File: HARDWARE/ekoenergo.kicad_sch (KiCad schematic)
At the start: 36 parts, among them J1 WSH500, J2 DC+, J3 EARTH, J4 DC-, J5 A, J6 B, Q1 47n60, Q2 47n60, Q3 47n60, Q4 47n60, U5 ACS712ELCTR-20A-T

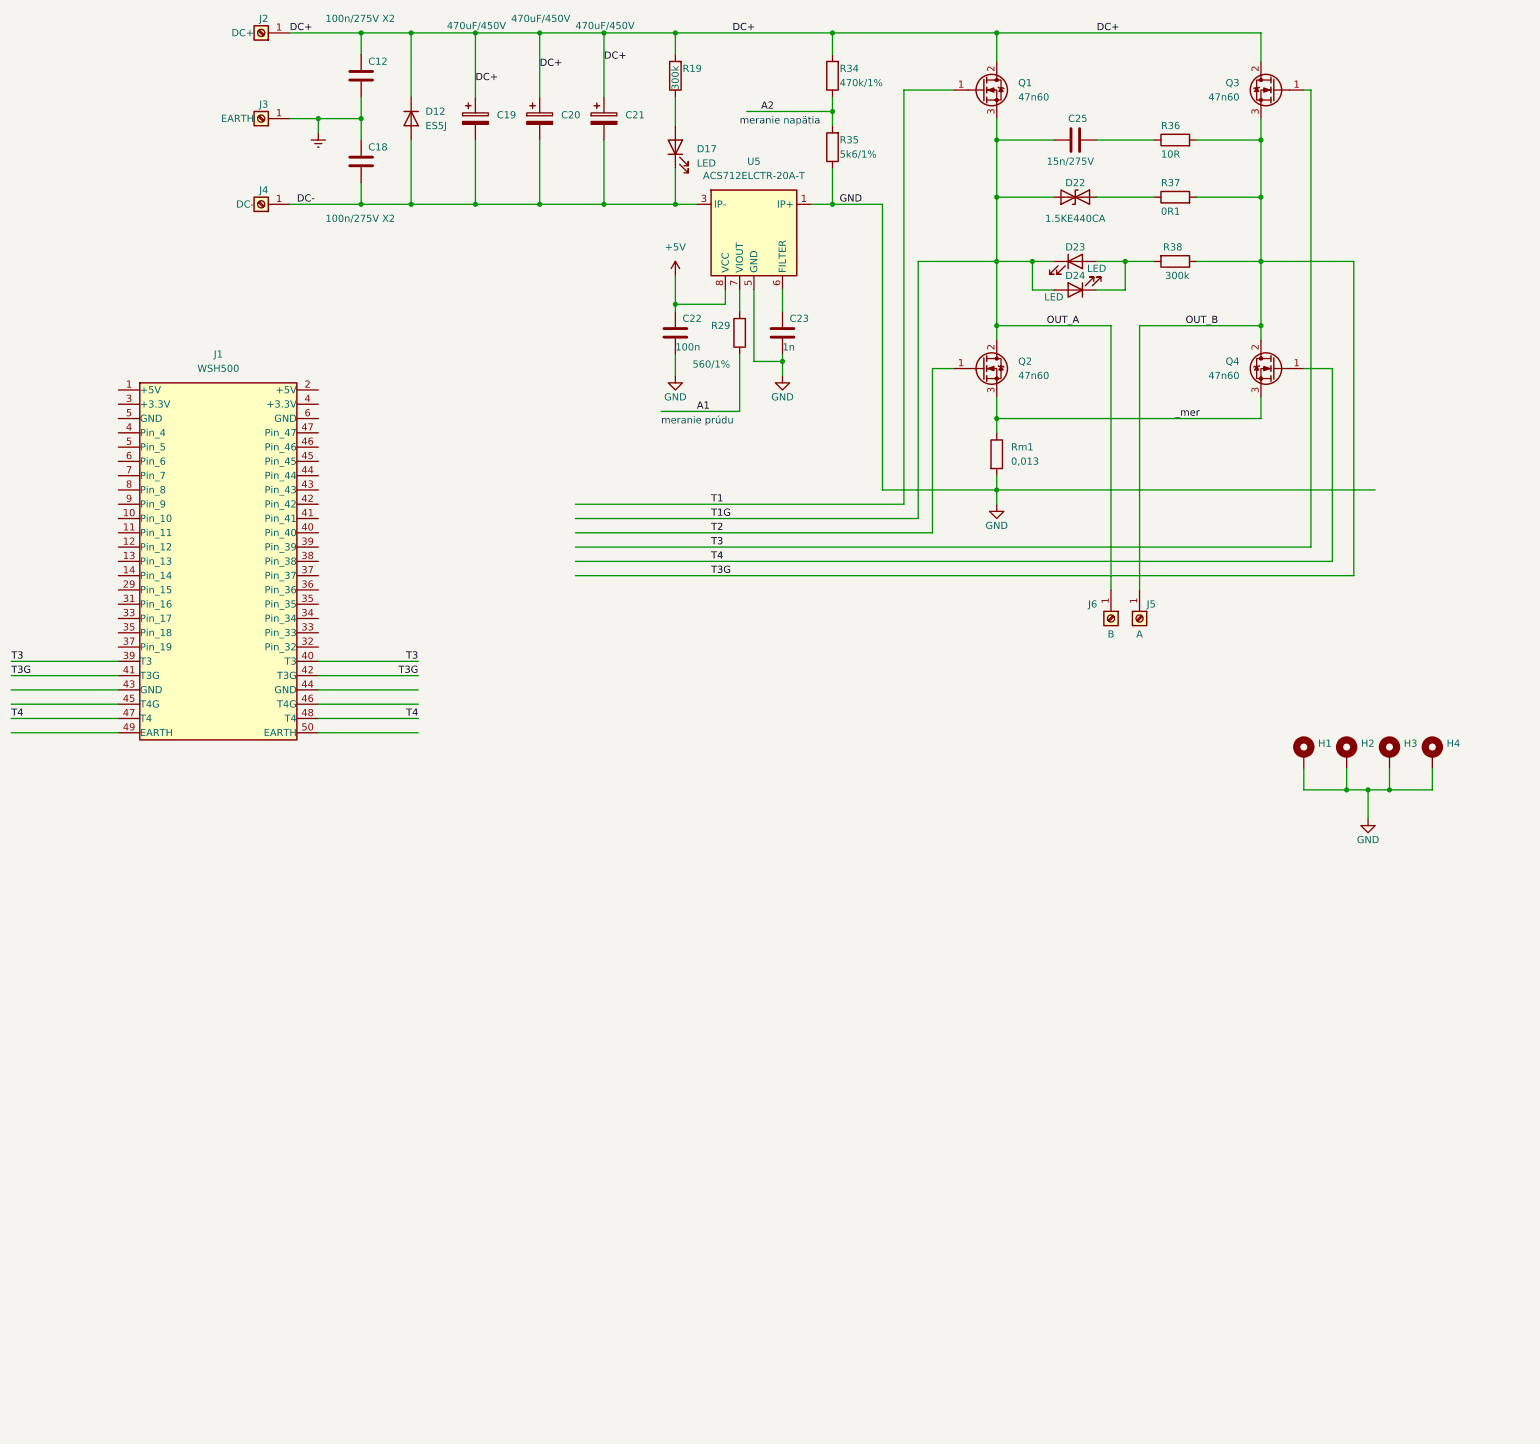
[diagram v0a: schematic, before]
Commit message: update
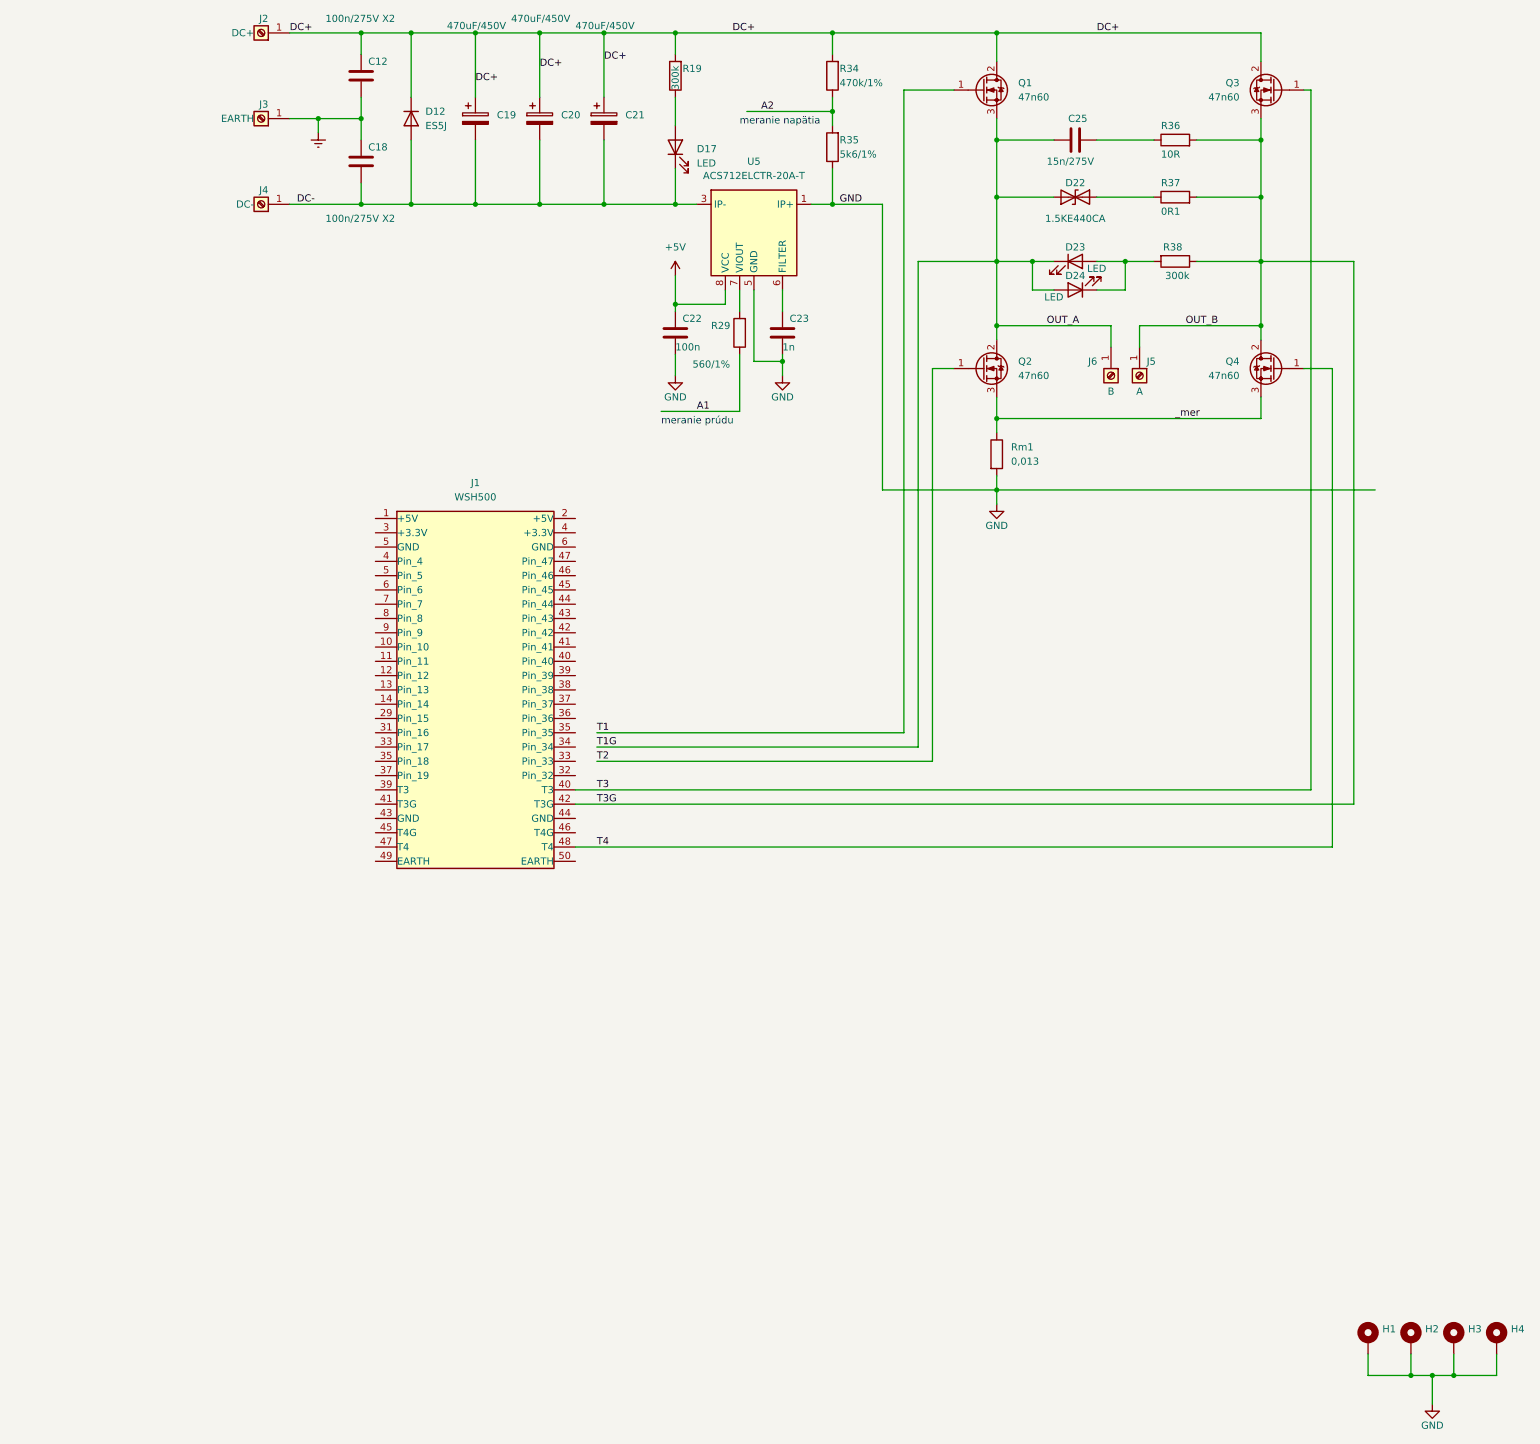
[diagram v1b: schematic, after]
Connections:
- net OUT_B: no longer J1.41 (Pin_41)
- net T3: no longer J1.39 (Pin_39)
- net T4: no longer J1.47 (Pin_47)
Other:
- moved on the sheet: H1, H2, H3, H4, J1, J5, J6
